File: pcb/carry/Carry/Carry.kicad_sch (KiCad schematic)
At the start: 7 parts, among them J2 Conn_01x02, U1 Luckfox-Pico_Mini_B, U2 MCP73831-2-OT

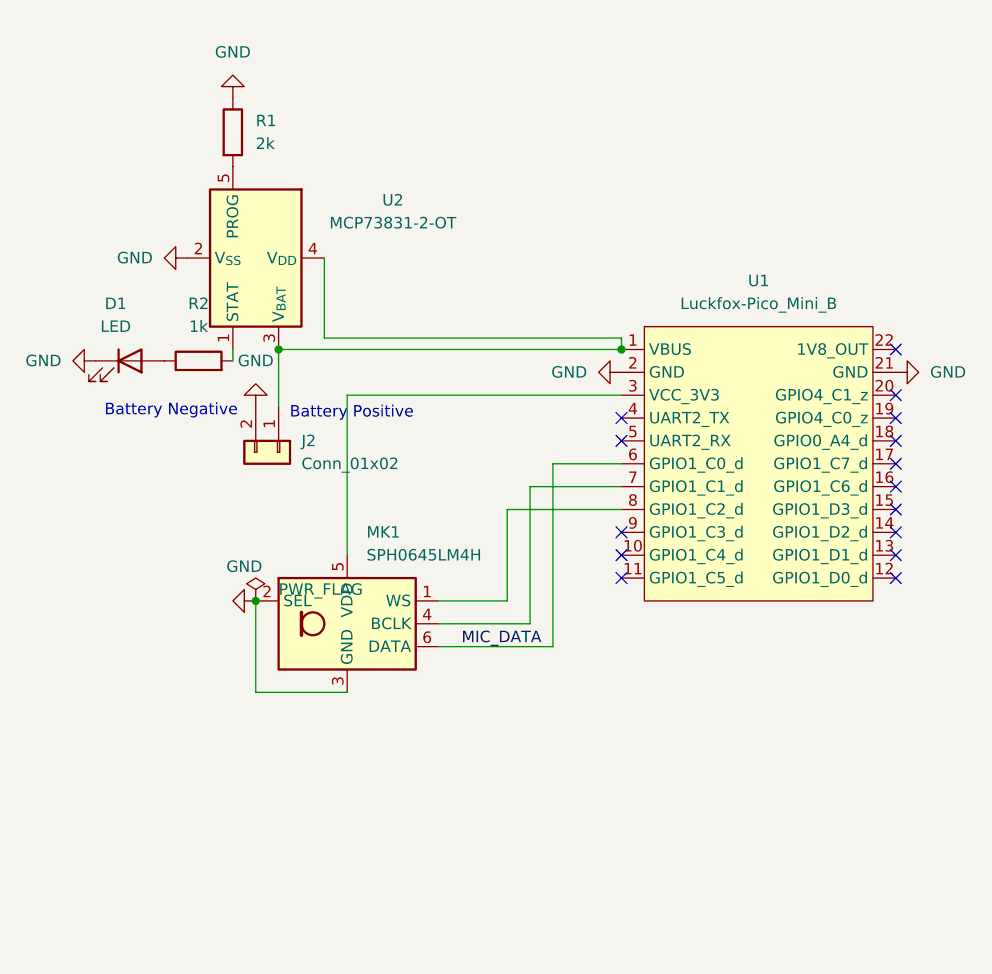
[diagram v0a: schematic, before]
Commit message: updated
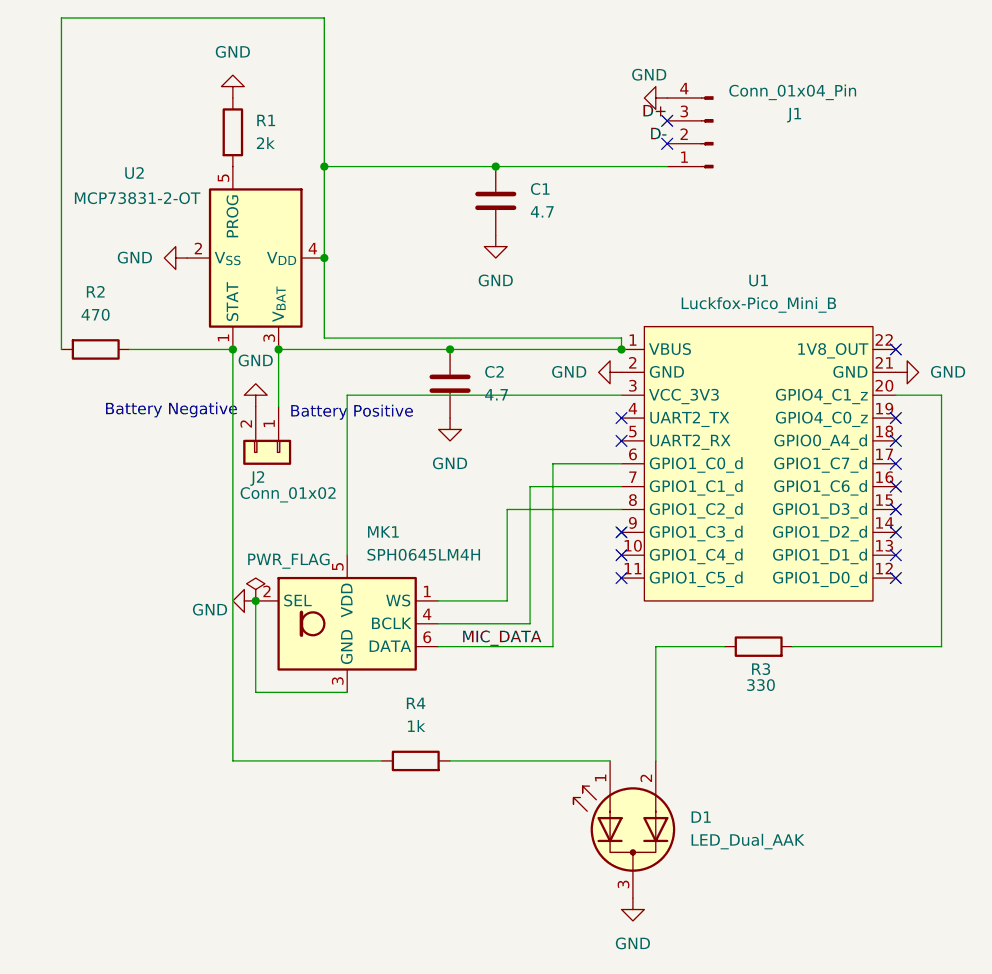
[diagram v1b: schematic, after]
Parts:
- removed D1: LED, symbol Device:LED
- added C1, C2: 4.7, symbol Device:C
- added D1: LED_Dual_AAK, LED_SMD:LED-L1T2_LUMILEDS, symbol Device:LED_Dual_AAK
- added J1: Conn_01x04_Pin, symbol Connector:Conn_01x04_Pin
- added R3: 330, symbol Device:R
- added R4: 1k, symbol Device:R
- R2: value 1k -> 470
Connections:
- net GND: now also C1.2, C2.2, D1.3 (K), J1.4 (Pin_4)
- net at J2.1 (Pin_1), U1.1 (VBUS), U2.3 (V_{BAT})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: now also R2.2, C1.1, C2.1, J1.1 (Pin_1)
- net at U1.20 (GPIO4_C1_z): now also R3.2
- net at R2.1: now also U2.1 (STAT), R4.1
- new net: D1.1 (A1), R4.2
- new net: D1.2 (A2), R3.1
- new net D+: J1.3 (Pin_3)
- new net D-: J1.2 (Pin_2)
- no-connect marks 15 -> 16
